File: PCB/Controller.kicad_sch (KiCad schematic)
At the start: 143 parts, among them J1 Screw_Terminal_01x08, J2 Screw_Terminal_01x08, J3 PH, J4 Screw_Terminal_01x08, J5 I2C Aux, J6 One Wire, K1 TE_PCH-1xxx2M, K2 TE_PCH-1xxx2M, Q1 BCX56, Q2 BCX56, Q3 BCX56, Q4 BCX56, U1 WeMos S3 Mini, U10 MCP3208, U2 L7805, U3 MIC5504-3.3YM5, U4 MIC5504-3.3YM5, U5 OPA2991, U6 MCP3021, U7 ISO1640BDR, U8 MC34072, U9 TL431D

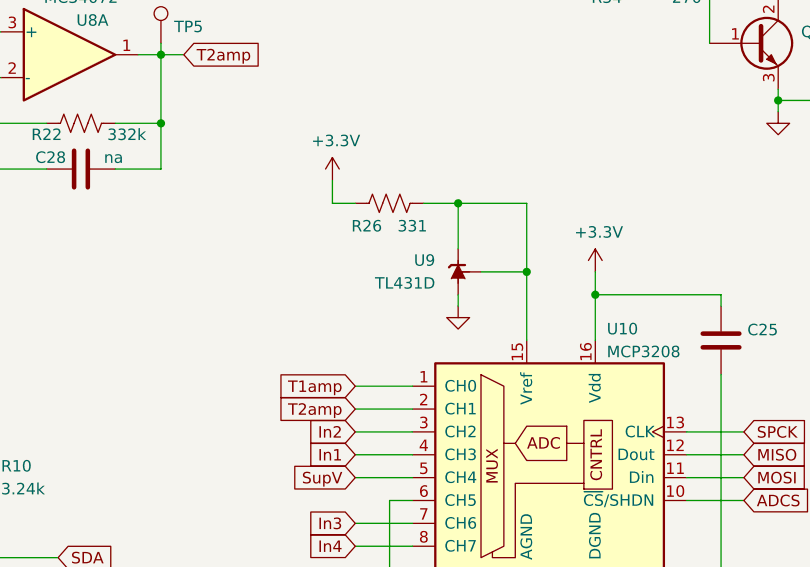
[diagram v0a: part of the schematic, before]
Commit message: Update to MBMon
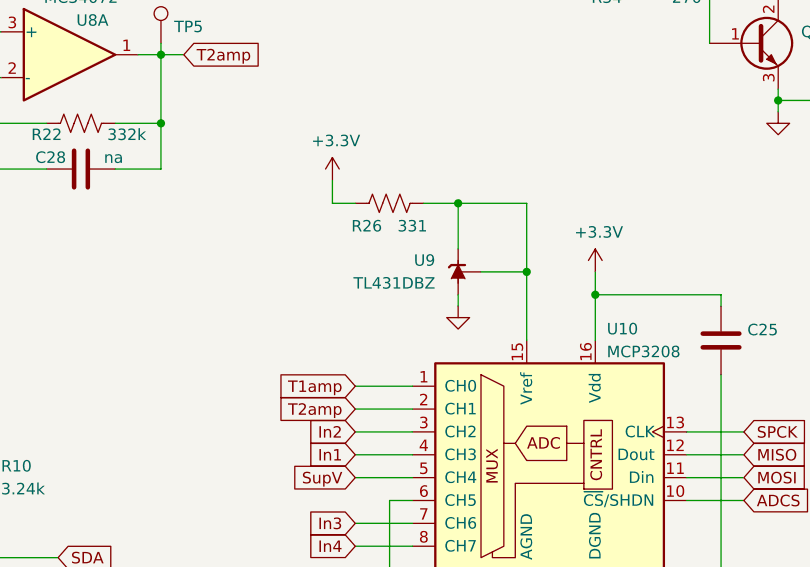
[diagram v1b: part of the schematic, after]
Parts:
- removed U9: TL431D, Package_SO:SOIC-8_3.9x4.9mm_P1.27mm, symbol Reference_Voltage:TL431D
- added U9: TL431DBZ, Package_TO_SOT_SMD:SOT-23, symbol Reference_Voltage:TL431DBZ
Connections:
- net GND: now also U9.3 (A)
- net at R26.2, U10.15 (Vref): now also U9.1 (K), U9.2 (REF)
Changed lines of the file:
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@@
+    )
+  )
+  (symbol (lib_id "Reference_Voltage:TL431DBZ") (at 274.32 189.23 270) (mirror x) (unit 1)
+    (in_bom yes) (on_board yes) (dnp no) (fields_autoplaced)
+    (property "Reference" "U9" (at 271.78 187.96 90)
+      (effects (font (size 1.27 1.27)) (justify right))
+    )
+    (property "Value" "TL431DBZ" (at 271.78 190.5 90)
+      (effects (font (size 1.27 1.27)) (justify right))
+    )
+    (property "Footprint" "Package_TO_SOT_SMD:SOT-23" (at 270.51 189.23 0)
+      (effects (font (size 1.27 1.27) italic) hide)
+    )
+    (property "Datasheet" "http://www.ti.com/lit/ds/symlink/tl431.pdf" (at 274.32 189.23 0)
+      (effects (font (size 1.27 1.27) italic) hide)
+    )
+    (pin "1")
+    (pin "2")
+    (pin "3")
+    (instances
+      (project "Controller"
+        (path "/e98a57d9-3732-4e84-8c7e-17ff22fc8918"
+          (reference "U9") (unit 1)
+        )
+      )
     )
   )
@@
         )
       )
-    )
-  )
-  (symbol (lib_id "Reference_Voltage:TL431D") (at 274.32 189.23 270) (mirror x) (unit 1)
-    (in_bom yes) (on_board yes) (dnp no) (fields_autoplaced)
-    (property "Reference" "U9" (at 271.78 187.96 90)
-      (effects (font (size 1.27 1.27)) (justify right))
-    )
-    (property "Value" "TL431D" (at 271.78 190.5 90)
-      (effects (font (size 1.27 1.27)) (justify right))
-    )
-    (property "Footprint" "Package_SO:SOIC-8_3.9x4.9mm_P1.27mm" (at 267.97 189.23 0)
-      (effects (font (size 1.27 1.27) italic) hide)
-    )
-    (property "Datasheet" "http://www.ti.com/lit/ds/symlink/tl431.pdf" (at 274.32 189.23 0)
-      (effects (font (size 1.27 1.27) italic) hide)
-    )
-    (pin "1")
-    (pin "2")
-    (pin "3")
-    (pin "6")
-    (pin "7")
-    (pin "8")
-    (instances
-      (project "Controller"
-        (path "/e98a57d9-3732-4e84-8c7e-17ff22fc8918"
-          (reference "U9") (unit 1)
-        )
-      )
